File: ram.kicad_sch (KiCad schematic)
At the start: 31 parts, among them SW3 SW_DIP_x08, SW4 SW_Push, U24 74189, U25 74189, U26 74LS157, U27 74LS157, U28 74LS04, U29 74LS04, U30 74LS245, U31 74LS00, U32 74LS157

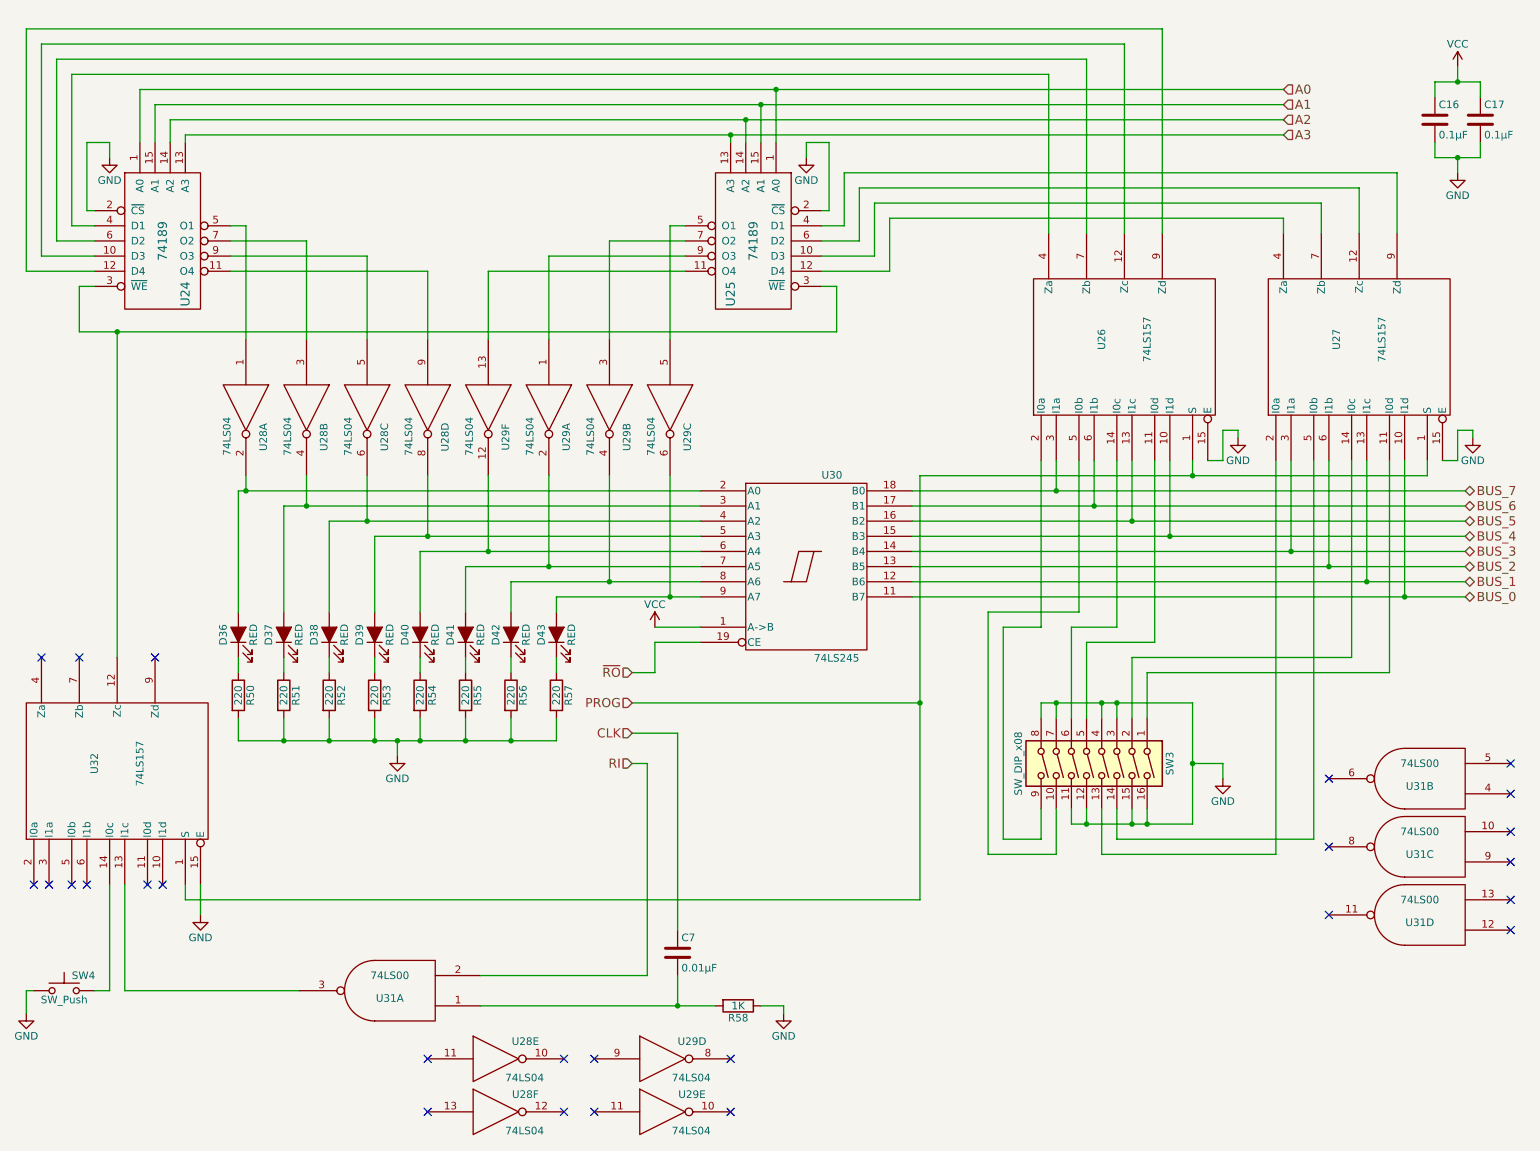
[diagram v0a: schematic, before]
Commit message: Add files via upload
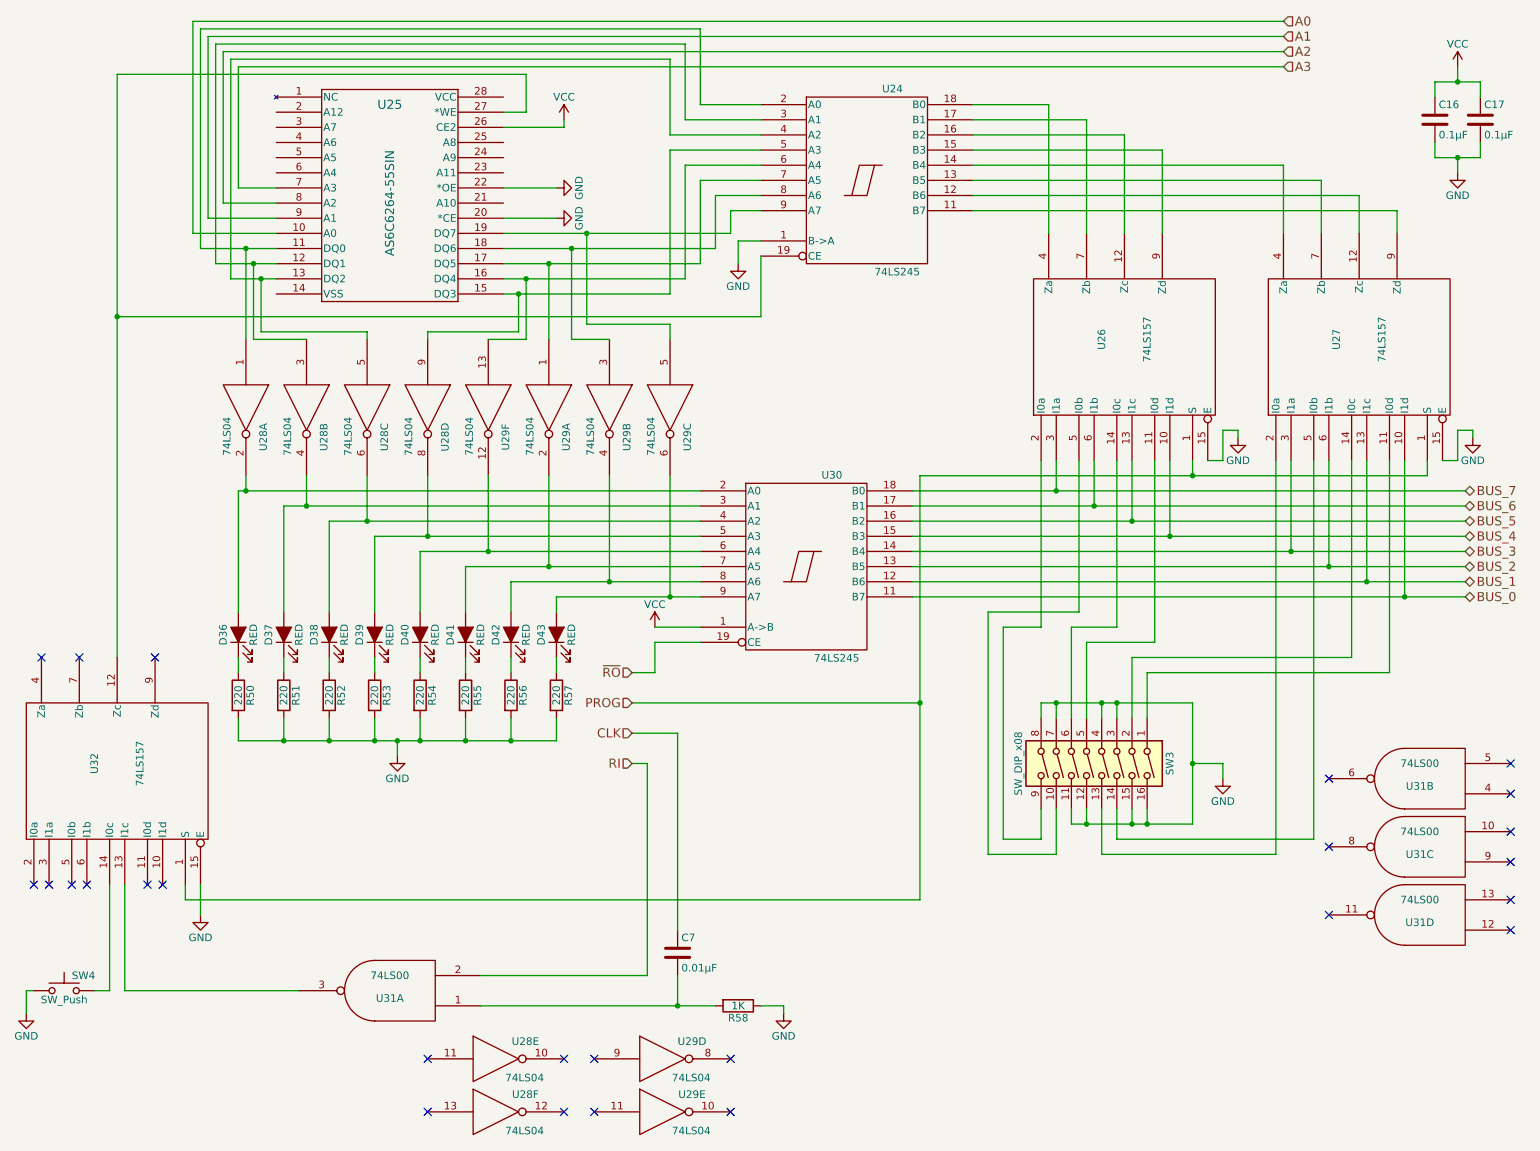
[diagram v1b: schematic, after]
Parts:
- removed U24, U25: 74189, Package_DIP:DIP-16_W7.62mm, symbol 8bit-computer-rescue:74189-8bit-computer-rescue
- added U24: 74LS245, Package_DIP:DIP-20_W7.62mm, symbol 8bit-computer-rescue:74LS245-8bit-computer-rescue
- added U25: AS6C6264-55SIN, SOP-28_MIL330_ALL, symbol AS6C264:AS6C6264-55SIN
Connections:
- net A0: now also U25.10 (A0)
- net A1: now also U25.9 (A1)
- net A2: now also U25.8 (A2)
- net A3: now also U25.7 (A3)
- net GND: now also U24.1 (B->A), U24.10 (GND), U25.20 (*CE), U25.22 (*OE)
- net VCC: now also U24.20 (VCC), U25.26 (CE2)
- net at U26.12 (Zc): now also U24.16 (B2)
- net at U28.9: now also U24.5 (A3), U25.15 (DQ3)
- net at U26.9 (Zd): now also U24.15 (B3)
- net at U32.12 (Zc): now also U24.19 (CE), U25.27 (*WE)
- net at U26.4 (Za): now also U24.18 (B0)
- net at U28.1: now also U24.2 (A0), U25.11 (DQ0)
- net at U26.7 (Zb): now also U24.17 (B1)
- net at U28.3: now also U24.3 (A1), U25.12 (DQ1)
- net at U28.5: now also U24.4 (A2), U25.13 (DQ2)
- net at U27.7 (Zb): now also U24.13 (B5)
- net at U29.13: now also U24.6 (A4), U25.16 (DQ4)
- net at U27.4 (Za): now also U24.14 (B4)
- net at U27.9 (Zd): now also U24.11 (B7)
- net at U29.5: now also U24.9 (A7), U25.19 (DQ7)
- net at U27.12 (Zc): now also U24.12 (B6)
- net at U29.3: now also U24.8 (A6), U25.18 (DQ6)
- net at U29.1: now also U24.7 (A5), U25.17 (DQ5)
